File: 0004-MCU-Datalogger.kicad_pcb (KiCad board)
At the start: 2 copper layers, 29 parts, among them J1 Conn_01x04_Pin, J2 Conn_01x04_Pin, J3 Conn_01x09_Pin, J4 Conn_02x03_Odd_Even, U1 24LC1025, U2 24LC1025, U3 DS1337S_, U4 ATMEGA328P-AU, Y1 16 MHz, Y2 32.768 KHz

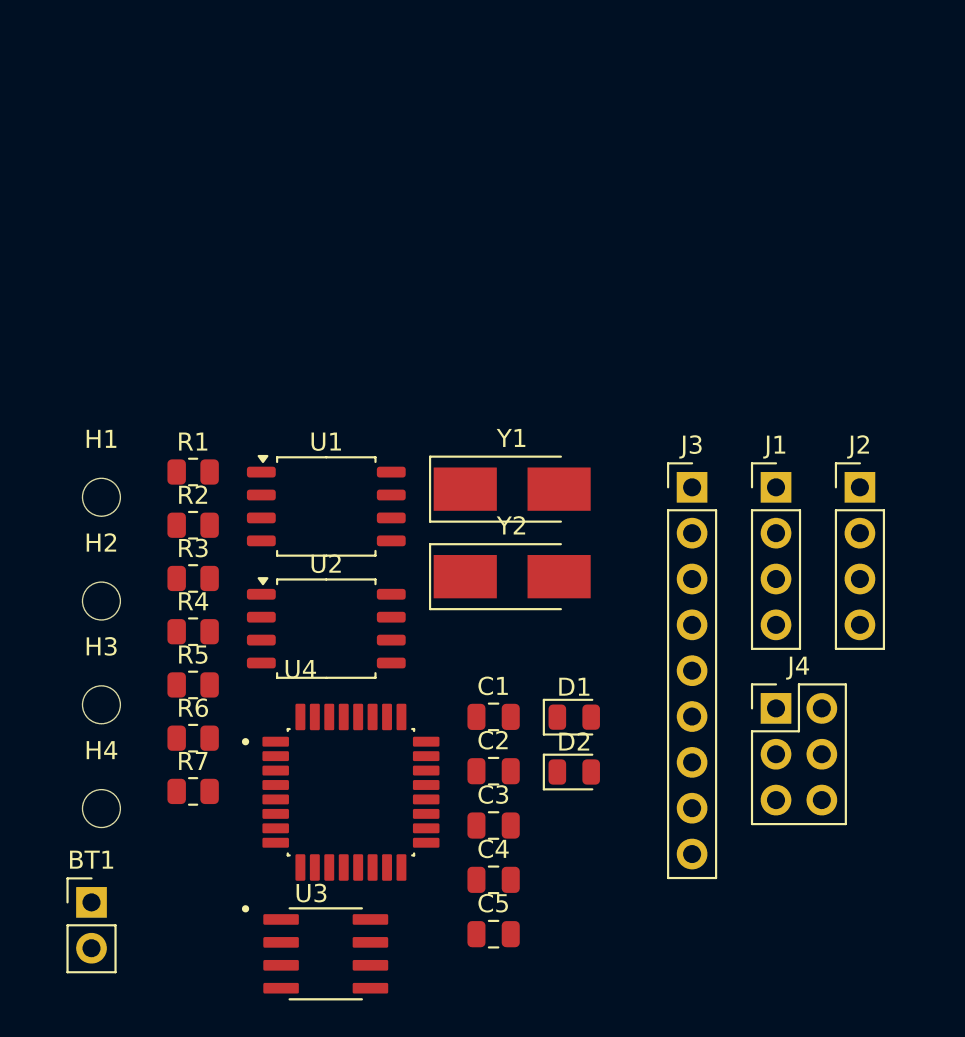
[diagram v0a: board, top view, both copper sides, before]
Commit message: Complete placement of footprints
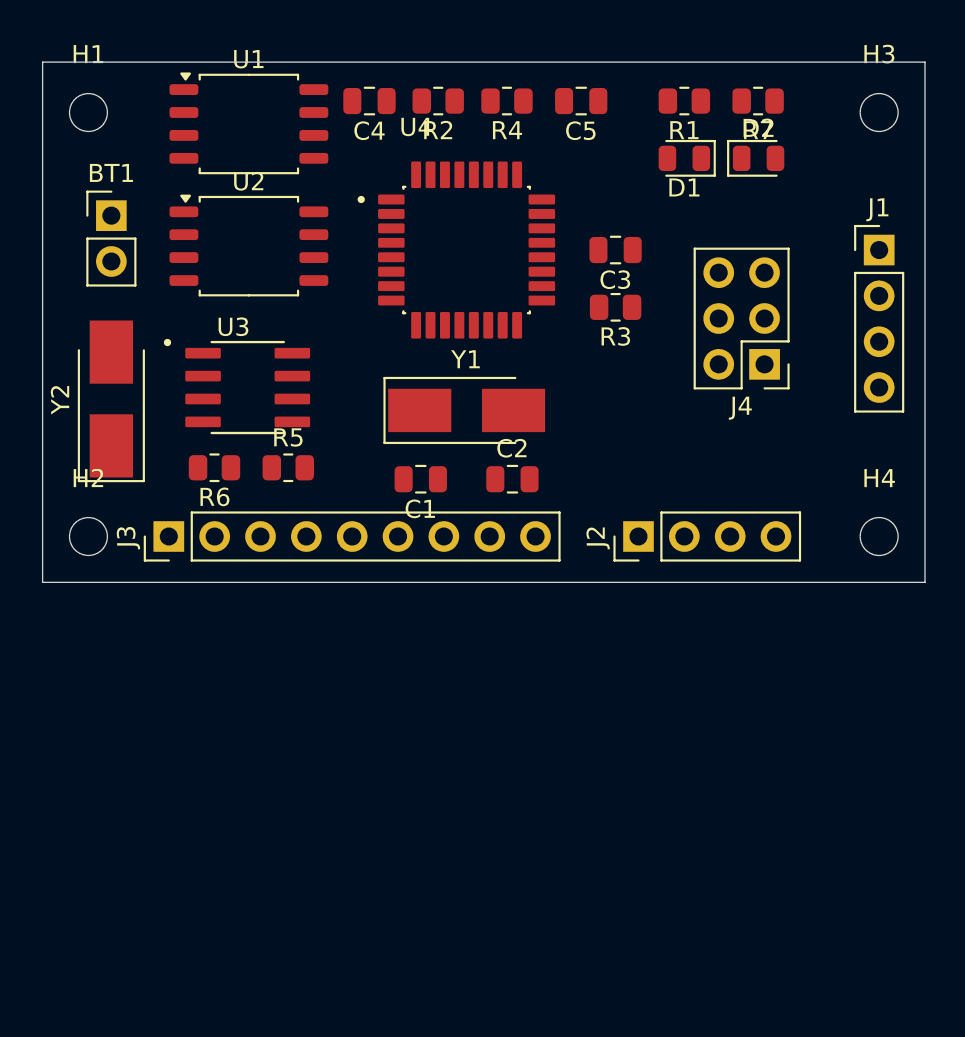
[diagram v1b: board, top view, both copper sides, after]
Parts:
- moved H3 54.2 mm to (167.0, 62.2)
- moved R7 49.4 mm to (160.3, 61.6), turned to 180 degrees
- moved C5 46.4 mm to (150.5, 61.6), turned to 180 degrees
- moved H4 45.7 mm to (167.0, 85.7)
- moved C4 43.7 mm to (138.8, 61.6), turned to 180 degrees
- moved BT1 38.1 mm to (124.5, 67.9)
- moved D2 35.5 mm to (160.3, 64.8)
- moved R4 34.2 mm to (146.4, 61.6), turned to 180 degrees
- moved R1 34.1 mm to (156.2, 61.6), turned to 180 degrees
- moved C3 32.6 mm to (152.4, 69.8), turned to 180 degrees
- moved U3 31.7 mm to (132.0, 77.5)
- moved D1 31.6 mm to (156.2, 64.8), turned to 180 degrees
- moved U4 30.7 mm to (144.1, 69.8)
- moved J3 29.1 mm to (127.6, 85.7), turned to 90 degrees
- moved R3 27.8 mm to (152.4, 73.0), turned to 180 degrees
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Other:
- board outline added: 48.9 x 28.8 mm

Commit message: Finish routing
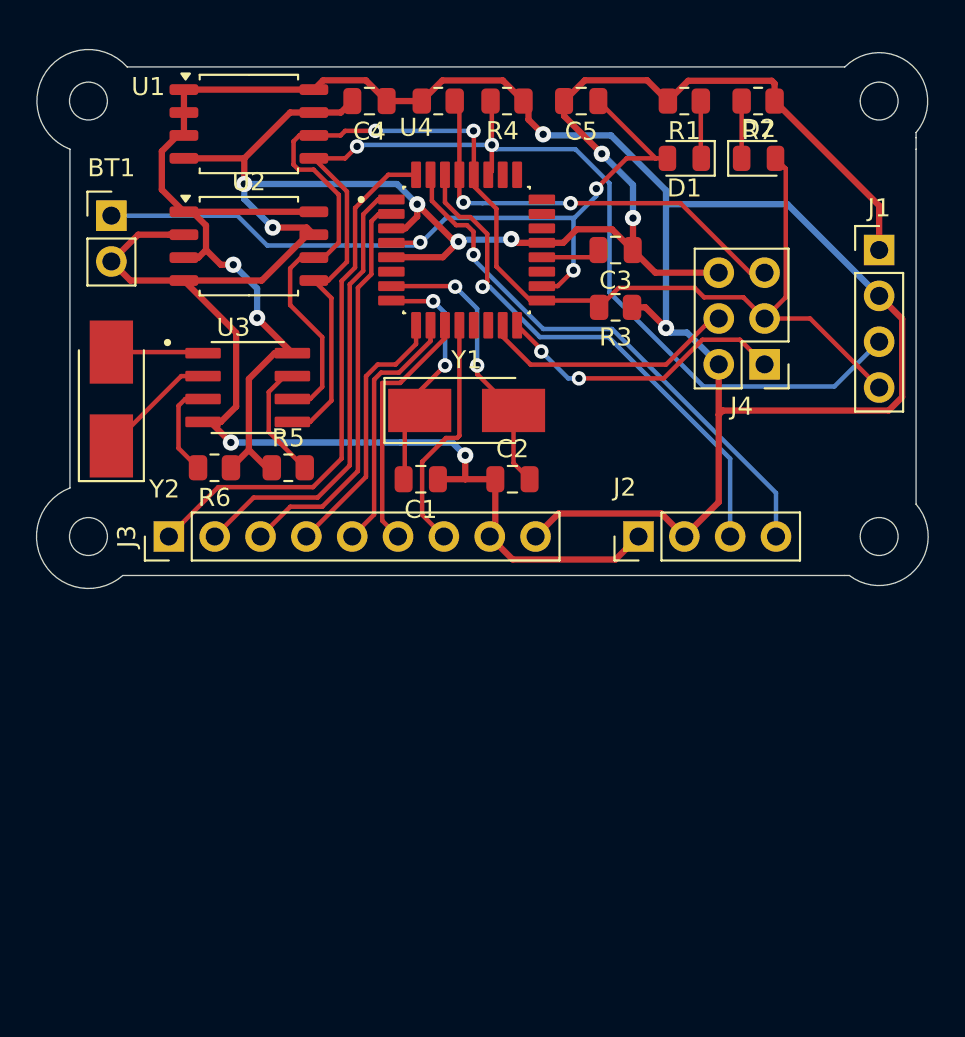
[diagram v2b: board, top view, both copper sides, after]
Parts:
- moved H1 0.63 mm to (123.2, 61.6)
- moved H3 0.63 mm to (167.0, 61.6)
- turned R2 to 0 degrees
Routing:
- net GND: track 0.00 -> 148.6 mm, vias 0 -> 9
- net /Vcc: track 0.00 -> 132.1 mm, vias 0 -> 4
- net /SCL: track 0.00 -> 72.3 mm, vias 0 -> 2
- net /SDA: track 0.00 -> 64.4 mm, vias 0 -> 2
- net Net-(BT1-+): track 0.00 -> 44.9 mm, vias 0 -> 3
- net /TX: track 0.00 -> 30.4 mm, vias 0 -> 1
- net /D2: track 0.00 -> 29.7 mm
- net /RX: track 0.00 -> 29.6 mm, vias 0 -> 1
- net /D3: track 0.00 -> 25.2 mm
- net /RESET: track 0.00 -> 24.1 mm, vias 0 -> 2
- net /D4: track 0.00 -> 22.3 mm
- net /MISO: track 0.00 -> 16.4 mm, vias 0 -> 2
- net Net-(U4-PB6): track 0.00 -> 15.9 mm, vias 0 -> 2
- net /D5: track 0.00 -> 14.8 mm
- net /MOSI: track 0.00 -> 14.3 mm
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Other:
- board size 48.9 x 28.8 mm -> 49.4 x 29.9 mm
